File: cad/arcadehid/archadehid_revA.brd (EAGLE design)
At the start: 160 x 100 mm, 30 parts, among them IC1 STM32F10XCXT6, IC3 AMS1117-3.3, X1 8MHz, X2 32.768kHz, X3 USB-MINIB

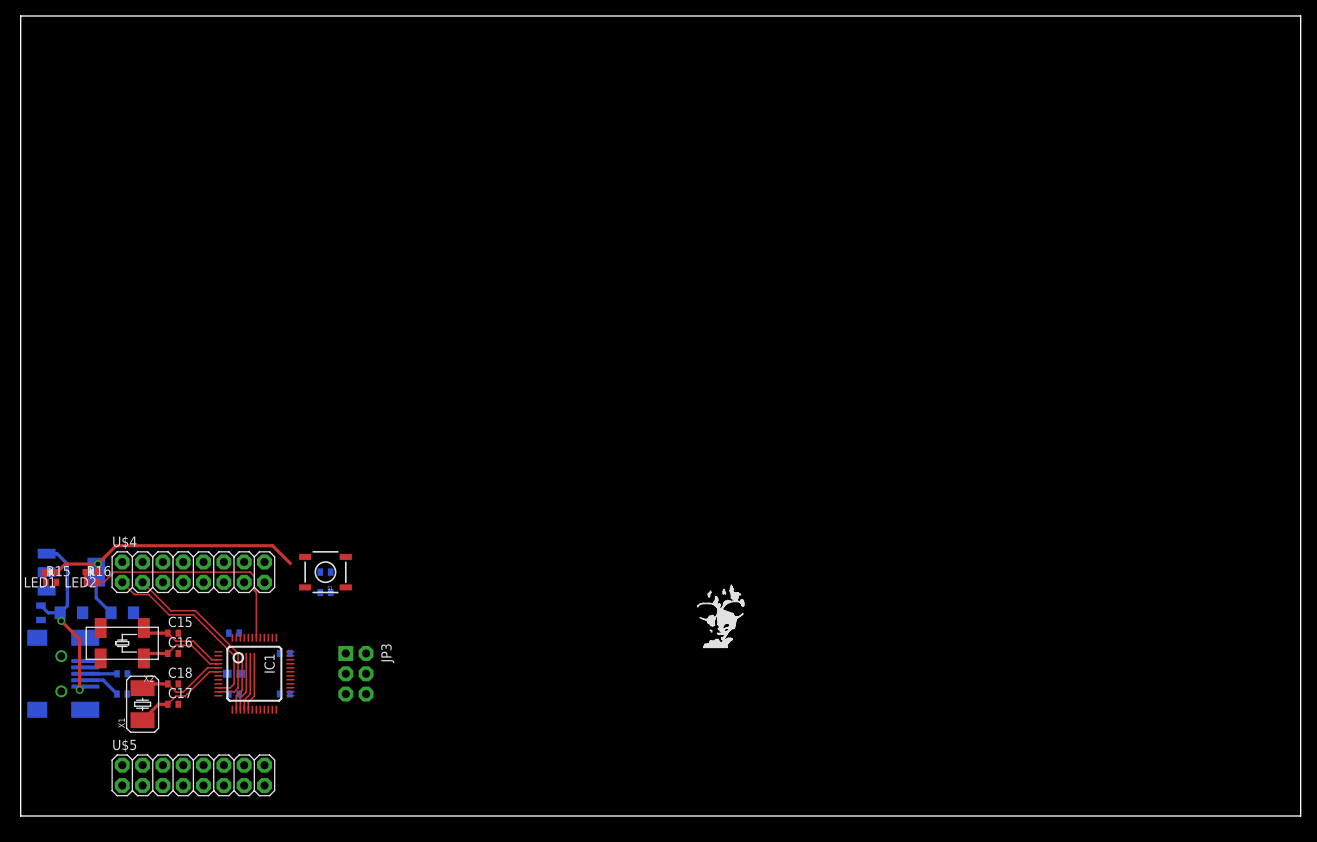
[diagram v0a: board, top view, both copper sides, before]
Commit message: cadding, almost there
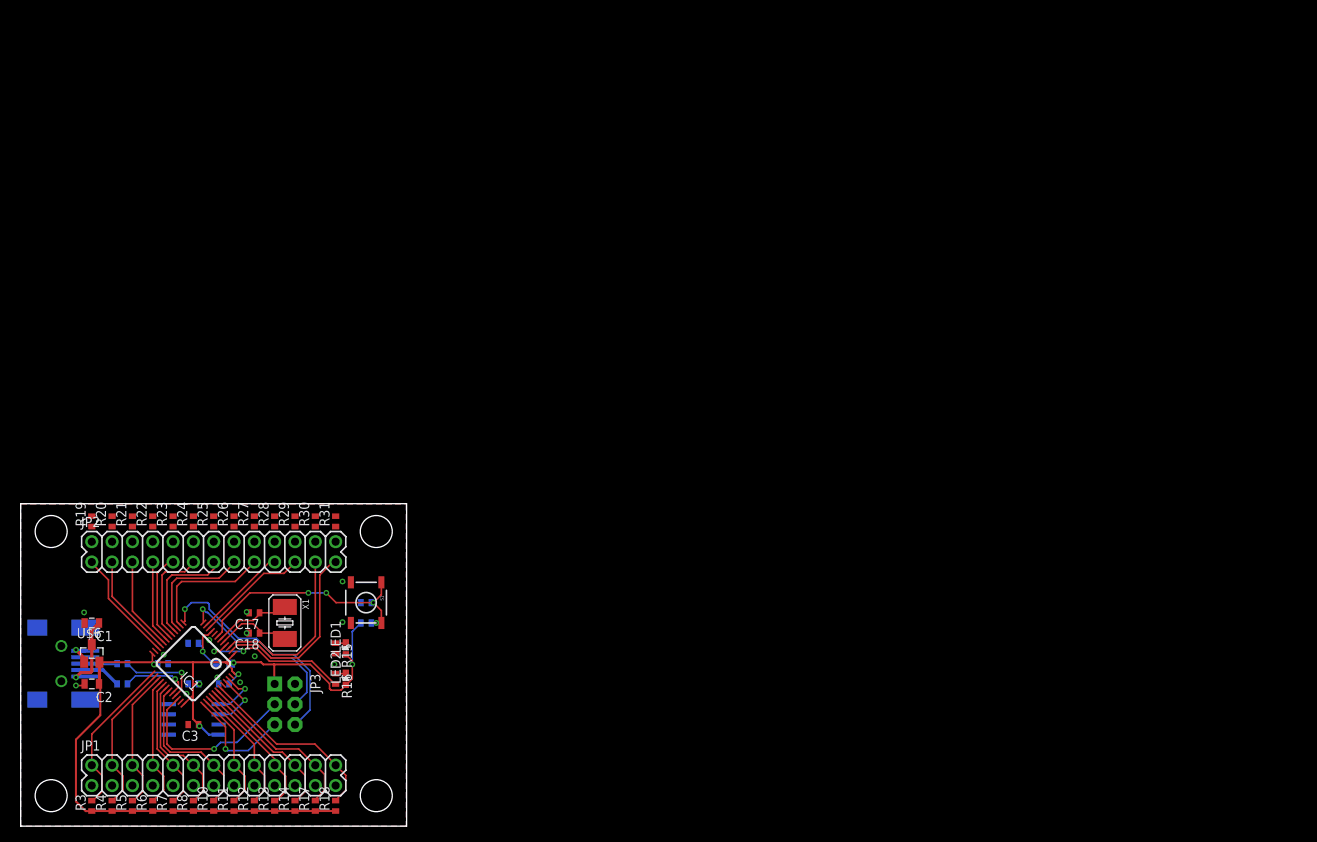
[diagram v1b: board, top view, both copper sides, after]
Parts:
- removed C15, C16: 24pF, robot:C0402
- removed C4: 1uF, robot:0805_GEN
- removed C5: 22uF, robot:EIA3216
- removed C7: 10uF, robot:EIA3216
- removed IC3: AMS1117-3.3, SparkFunEagle-6-6-07:SOT223
- removed U$4, U$5: M08X2, SparkFun-Connectors:2X8
- removed X2: 32.768kHz, robot:CRYSTAL_SMD_8X4_ACT
- added C1, C2: 1uF, robot:0805_GEN
- added C3: 0.1uF, robot:C0402
- added JP1, JP2: M13X22X13, SparkFun-Connectors:2X13
- added R10, R11, R12, R13, R14, R17, R18, R19, R20, R21, R22, R23, R24, R25, R26, R27, R28, R29, R3, R30, R31, R4, R5, R6, R7, R8: 30k, SparkFunEagle-6-6-07:C0402
- added U$2: MEMORYI2COWN, robot:SO-8
- added U$6: XC6206OWNOWN, robot:SOT23
- moved U$7 44.9 mm to (44.0, 14.7), flipped to the bottom
- moved LED1 38.0 mm to (40.6, 21.0), turned to 0 degrees
- moved R15 36.5 mm to (39.4, 21.0), turned to 270 degrees
- moved LED2 34.4 mm to (40.6, 17.1), turned to 0 degrees
- moved R16 32.8 mm to (39.4, 17.1), turned to 270 degrees
- moved X1 20.5 mm to (33.0, 24.1), turned to 270 degrees
- moved C10 15.7 mm to (17.8, 19.1), turned to 180 degrees
- moved C17 15.3 mm to (29.2, 25.4), turned to 180 degrees
- moved C18 12.0 mm to (29.2, 22.9), turned to 180 degrees
- moved JP3 9.67 mm to (33.0, 14.0)
- moved C11 8.52 mm to (25.4, 16.5), turned to 0 degrees
- moved C13 8.13 mm to (21.6, 21.6)
- moved C12 8.13 mm to (21.6, 16.5), turned to 0 degrees
- moved IC1 7.73 mm to (21.6, 19.1), turned to 135 degrees
- moved R9 6.35 mm to (43.2, 24.1), turned to 180 degrees
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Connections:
- removed net I2C_SCL: IC1.21
- removed net IOEXP_INT: IC1.2
- removed net N$18: U$5.16
- removed net RADIO_TXEN: IC1.41
- removed net RANGE_SENS_PULS_H/JOY_VERT: IC1.18
- removed net RANGE_SENS_PULS_L/JOY_HORI: IC1.19
- removed net RTCI: C15.1, IC1.3, X2.P$1
- removed net RTCO: C16.1, IC1.4, X2.P$4
- removed net SERVO_PAN/SCR_VSYNC: IC1.45
- removed net SERVO_RANGE/JOY_BUTT: IC1.43
- removed net SERVO_TILT/HONK: IC1.46
- removed net TDI: IC1.38
- removed net TDO: IC1.39
- removed net TRST: IC1.40
- removed net VBAT_LOAD_EN: IC1.20
- new net PA15: IC1.38, JP1.16, R11.2
- new net PB0: IC1.18, JP2.9, R23.1
- new net PB1: IC1.19, JP2.7, R22.1
- new net PB10: IC1.21, JP2.3, R20.1
- new net PB2: IC1.20, JP2.5, R21.1
- new net PB3: IC1.39, JP1.18, R12.2
- new net PB4: IC1.40, JP1.20, R13.2
- new net PB5: IC1.41, JP1.22, R14.2
- new net PB6: IC1.42, JP1.24, R17.2
- new net PB7: IC1.43, JP1.26, R18.2
- new net PB8: IC1.45, U$2.6
- new net PB9: IC1.46, U$2.5
- new net PC13: IC1.2, JP2.25, R31.1
- new net PC14: IC1.3, JP2.23, R30.1
- net 3.3V: now also C2.1, C3.1, R10.1, R11.1, R12.1, R13.1, R14.1, R17.1, R18.1, R19.2, R20.2, R21.2, R22.2, R23.2, R24.2, R25.2, R26.2, R27.2, R28.2, R29.2, R3.1, R30.2, R31.2, R4.1, R5.1, R6.1, R7.1, R8.1, U$2.8, U$6.2; no longer C5.A, IC3.2, IC3.4
- net 5V: now also C1.1, U$6.3; no longer C4.1, C7.A, IC3.3
- net GND: now also C1.2, C2.2, C3.2, JP1.1, JP1.11, JP1.13, JP1.15, JP1.17, JP1.19, JP1.21, JP1.23, JP1.25, JP1.3, JP1.5, JP1.7, JP1.9, JP2.10, JP2.12, JP2.14, JP2.16, JP2.18, JP2.2, JP2.20, JP2.22, JP2.24, JP2.26, JP2.4, JP2.6, JP2.8, U$2.2, U$2.3, U$2.4, U$2.7, U$6.1; no longer C15.2, C16.2, C4.2, C5.C, C7.C, IC3.1
- net LED_A: now also IC1.4; no longer IC1.42
- net PA0: now also JP2.21, R29.1; no longer U$4.1
- net PA1: now also JP2.19, R28.1; no longer U$4.3
- net PA10: now also JP1.14, R10.2; no longer U$5.6
- net PA4: now also JP2.17, R27.1; no longer U$4.9
- net PA5: now also JP2.15, R26.1; no longer U$4.11
- net PA6: now also JP2.13, R25.1; no longer U$4.13
- net PA7: now also JP2.11, R24.1; no longer U$4.15
- net PA8: now also JP1.10, R7.2; no longer U$5.2
- net PA9: now also JP1.12, R8.2; no longer U$5.4
- net PB11: now also JP2.1, R19.1; no longer U$5.8
- net PB12: now also JP1.2, R3.2; no longer U$5.10
- net PB13: now also JP1.4, R4.2; no longer U$5.12
- net PB14: now also JP1.6, R5.2; no longer U$5.14
- net PB15: now also JP1.8, R6.2
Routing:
- net 3.3V: track 39.4 -> 120.2 mm, vias 1 -> 6
- net RST: track 0.00 -> 30.5 mm, vias 0 -> 4
- net USART_RX: track 0.00 -> 29.1 mm, vias 0 -> 1
- net PB7: track 0.00 -> 23.9 mm
- net PC13: track 0.00 -> 23.5 mm
- net USART_TX: track 0.00 -> 22.6 mm, vias 0 -> 1
- net SWDIO: track 0.00 -> 22.3 mm, vias 0 -> 1
- net PC14: track 0.00 -> 22.1 mm
- net PB6: track 0.00 -> 21.5 mm
- net PB12: track 0.00 -> 20.2 mm
- net PA10: track 0.00 -> 20.0 mm
- net PB5: track 0.00 -> 19.4 mm
- net PB13: track 0.00 -> 18.9 mm
- net PA9: track 0.00 -> 18.2 mm
- net PB14: track 0.00 -> 17.6 mm
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- added copper zone on layer 1, net GND
- added copper zone on layer 16, net GND
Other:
- board size 160 x 100 mm -> 48.2 x 40.3 mm
